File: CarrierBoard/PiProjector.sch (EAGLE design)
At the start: 73 parts, among them P8 PINHEAD2X23, P9 PINHEAD2X23, Q1 BCX70SMD, X1 24MHz, X2 12Mhz

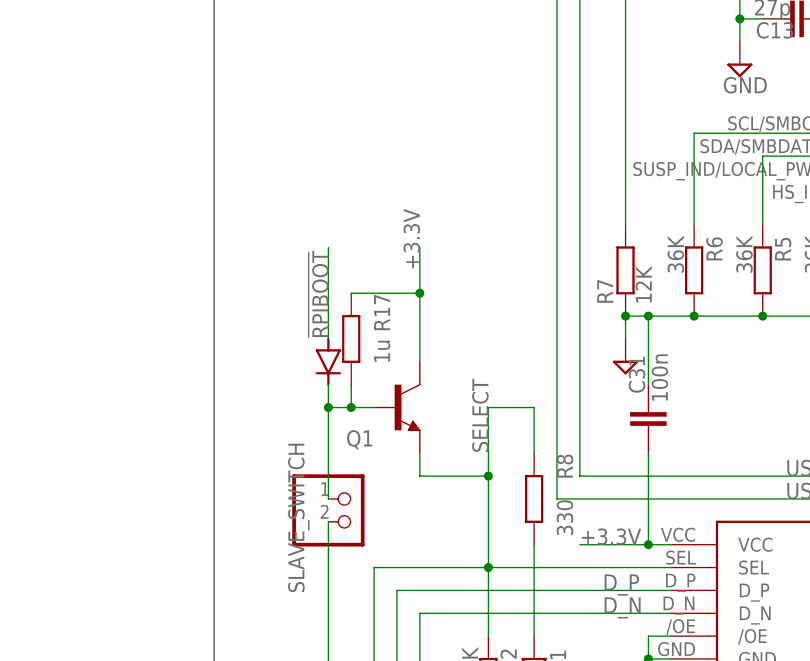
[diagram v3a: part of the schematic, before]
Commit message: Fixed rpiboot
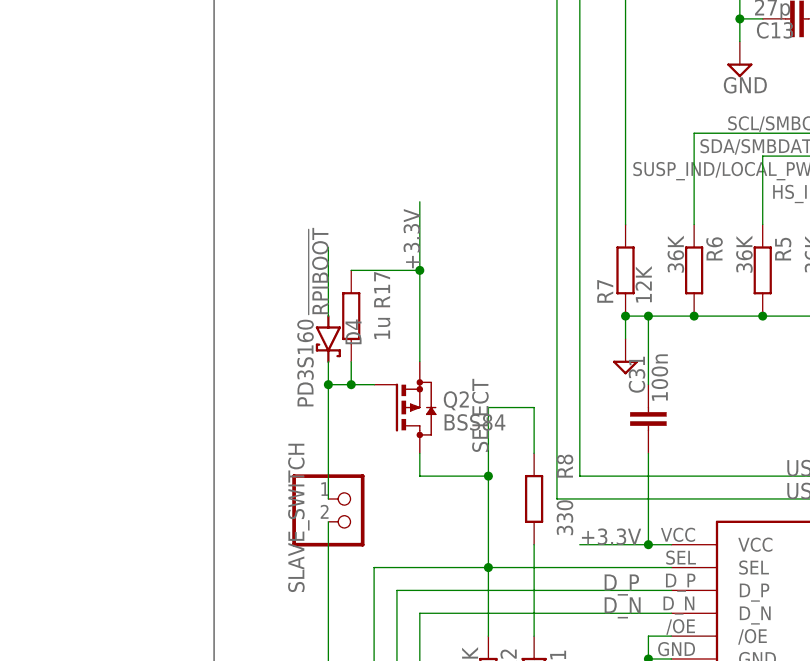
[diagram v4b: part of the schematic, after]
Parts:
- removed Q1: BCX70SMD, transistor-npn:BCX70SMD
- added D4: PD3S160, diode:PD3S160
- added Q2: BSS84, transistor-small-signal:BSS84
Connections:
- net !RPIBOOT: now also D4.A
- net +3.3V: now also Q2.S; no longer Q1.C
- net N$8: now also D4.C, Q2.G; no longer Q1.B
- net SELECT: now also Q2.D; no longer Q1.E
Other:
- moved on the sheet: R17
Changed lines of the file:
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@@
 <part name="SUPPLY29" library="supply2" library_urn="urn:adsk.eagle:library:372" deviceset="GND" device=""/>
 <part name="SUPPLY30" library="supply2" library_urn="urn:adsk.eagle:library:372" deviceset="GND" device=""/>
-<part name="Q1" library="transistor-npn" library_urn="urn:adsk.eagle:library:398" deviceset="BCX70*" device="SMD" package3d_urn="urn:adsk.eagle:package:28738/2"/>
 <part name="R17" library="pm-labs" deviceset="R" device="0603R" value="1u"/>
 <part name="SUPPLY5" library="supply2" library_urn="urn:adsk.eagle:library:372" deviceset="GND" device=""/>
 <part name="SUPPLY22" library="supply2" library_urn="urn:adsk.eagle:library:372" deviceset="GND" device=""/>
-<part name="D3" library="docu-dummy" library_urn="urn:adsk.eagle:library:215" deviceset="DIODE" device=""/>
+<part name="D4" library="diode" library_urn="urn:adsk.eagle:library:210" deviceset="PD3S160" device="" package3d_urn="urn:adsk.eagle:package:43459/1"/>
+<part name="Q2" library="transistor-small-signal" library_urn="urn:adsk.eagle:library:401" deviceset="BSS84" device="" package3d_urn="urn:adsk.eagle:package:28738/2"/>
 </parts>
 <sheets>
@@
 <attribute name="VALUE" x="-45.085" y="210.185" size="1.778" layer="96"/>
 </instance>
-<instance part="Q1" gate="G$1" x="147.32" y="195.58" smashed="yes">
-<attribute name="NAME" x="144.78" y="193.04" size="1.778" layer="95" rot="R180"/>
-</instance>
-<instance part="R17" gate="R" x="142.24" y="203.2" smashed="yes" rot="R270">
-<attribute name="NAME" x="144.78" y="208.28" size="1.778" layer="95" rot="R270"/>
-<attribute name="VALUE" x="144.78" y="203.2" size="1.778" layer="96" rot="R270"/>
+<instance part="R17" gate="R" x="142.24" y="205.74" smashed="yes" rot="R270">
+<attribute name="NAME" x="144.78" y="210.82" size="1.778" layer="95" rot="R270"/>
+<attribute name="VALUE" x="144.78" y="205.74" size="1.778" layer="96" rot="R270"/>
 </instance>
 <instance part="SUPPLY5" gate="GND" x="162.56" y="157.48" smashed="yes">
@@
 <attribute name="VALUE" x="137.795" y="154.305" size="1.778" layer="96"/>
 </instance>
-<instance part="D3" gate="G$1" x="139.7" y="200.66" smashed="yes" rot="R270"/>
+<instance part="D4" gate="G$1" x="139.7" y="203.2" smashed="yes" rot="R270">
+<attribute name="NAME" x="141.605" y="205.486" size="1.778" layer="95" rot="R270"/>
+<attribute name="VALUE" x="136.271" y="205.486" size="1.778" layer="96" rot="R270"/>
+</instance>
+<instance part="Q2" gate="G$1" x="149.86" y="195.58" smashed="yes">
+<attribute name="NAME" x="152.4" y="195.58" size="1.778" layer="95"/>
+<attribute name="VALUE" x="152.4" y="193.04" size="1.778" layer="96"/>
+</instance>
 </instances>
 <busses>
@@
 </segment>
 <segment>
-<pinref part="Q1" gate="G$1" pin="C"/>
-<wire x1="149.86" y1="208.28" x2="149.86" y2="200.66" width="0.1524" layer="91"/>
+<wire x1="149.86" y1="210.82" x2="149.86" y2="200.66" width="0.1524" layer="91"/>
 <pinref part="R17" gate="R" pin="1"/>
-<wire x1="149.86" y1="208.28" x2="142.24" y2="208.28" width="0.1524" layer="91"/>
-<junction x="149.86" y="208.28"/>
-<wire x1="149.86" y1="213.36" x2="149.86" y2="208.28" width="0.1524" layer="91"/>
+<wire x1="149.86" y1="210.82" x2="142.24" y2="210.82" width="0.1524" layer="91"/>
+<junction x="149.86" y="210.82"/>
 <label x="149.86" y="210.82" size="1.778" layer="95" rot="R90"/>
+<pinref part="Q2" gate="G$1" pin="S"/>
+<wire x1="149.86" y1="210.82" x2="149.86" y2="218.44" width="0.1524" layer="91"/>
 </segment>
 </net>
@@
 </segment>
 <segment>
-<wire x1="139.7" y1="203.2" x2="139.7" y2="213.36" width="0.1524" layer="91"/>
-<label x="139.7" y="203.2" size="1.778" layer="95" rot="R90"/>
+<wire x1="139.7" y1="205.74" x2="139.7" y2="213.36" width="0.1524" layer="91"/>
+<label x="139.7" y="205.74" size="1.778" layer="95" rot="R90"/>
+<pinref part="D4" gate="G$1" pin="A"/>
 </segment>
 </net>
@@
 <wire x1="157.48" y1="195.58" x2="157.48" y2="187.96" width="0.1524" layer="91"/>
 <label x="157.48" y="190.5" size="1.778" layer="95" rot="R90"/>
-<pinref part="Q1" gate="G$1" pin="E"/>
 <wire x1="157.48" y1="187.96" x2="157.48" y2="177.8" width="0.1524" layer="91"/>
 <wire x1="149.86" y1="190.5" x2="149.86" y2="187.96" width="0.1524" layer="91"/>
 <wire x1="149.86" y1="187.96" x2="157.48" y2="187.96" width="0.1524" layer="91"/>
 <junction x="157.48" y="187.96"/>
+<pinref part="Q2" gate="G$1" pin="D"/>
 </segment>
 </net>
@@
 <segment>
 <pinref part="R17" gate="R" pin="2"/>
-<wire x1="142.24" y1="198.12" x2="142.24" y2="195.58" width="0.1524" layer="91"/>
-<pinref part="Q1" gate="G$1" pin="B"/>
-<wire x1="142.24" y1="195.58" x2="144.78" y2="195.58" width="0.1524" layer="91"/>
-<wire x1="142.24" y1="195.58" x2="139.7" y2="195.58" width="0.1524" layer="91"/>
-<wire x1="139.7" y1="195.58" x2="139.7" y2="185.42" width="0.1524" layer="91"/>
-<junction x="142.24" y="195.58"/>
+<wire x1="142.24" y1="200.66" x2="142.24" y2="198.12" width="0.1524" layer="91"/>
+<wire x1="142.24" y1="198.12" x2="144.78" y2="198.12" width="0.1524" layer="91"/>
+<wire x1="142.24" y1="198.12" x2="139.7" y2="198.12" width="0.1524" layer="91"/>
+<wire x1="139.7" y1="198.12" x2="139.7" y2="185.42" width="0.1524" layer="91"/>
+<junction x="142.24" y="198.12"/>
 <pinref part="SLAVE_SWITCH" gate="G$1" pin="1"/>
-<wire x1="139.7" y1="195.58" x2="139.7" y2="198.12" width="0.1524" layer="91"/>
-<junction x="139.7" y="195.58"/>
-</segment>
-</net>
+<wire x1="139.7" y1="198.12" x2="139.7" y2="200.66" width="0.1524" layer="91"/>
+<junction x="139.7" y="198.12"/>
+<pinref part="D4" gate="G$1" pin="C"/>
+<pinref part="Q2" gate="G$1" pin="G"/>
+</segment>
+</net>

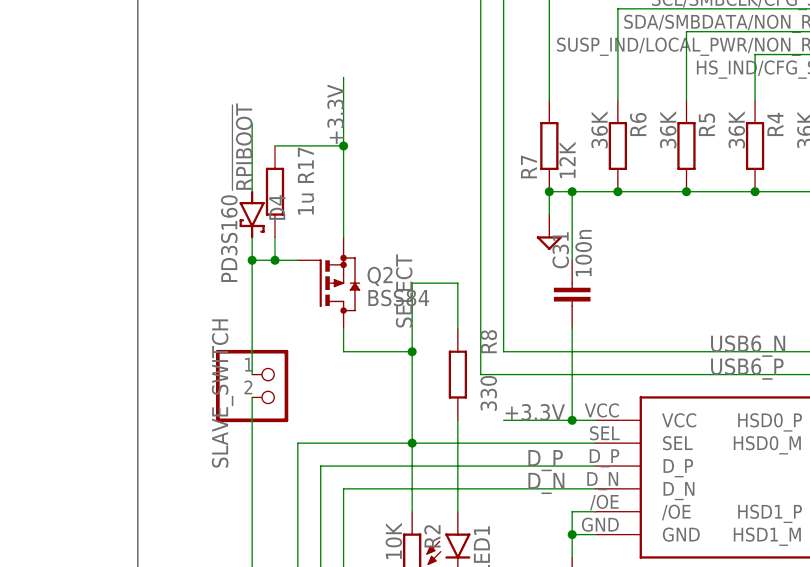
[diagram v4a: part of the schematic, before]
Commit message: Fixed RPI and USB switch Pulldown
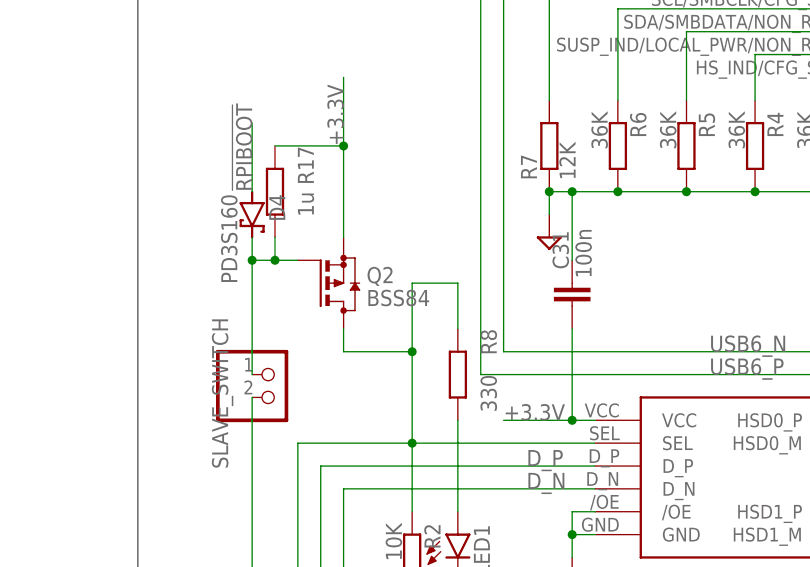
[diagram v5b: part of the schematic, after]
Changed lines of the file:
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@@
 <wire x1="157.48" y1="195.58" x2="162.56" y2="195.58" width="0.1524" layer="91"/>
 <wire x1="157.48" y1="195.58" x2="157.48" y2="187.96" width="0.1524" layer="91"/>
-<label x="157.48" y="190.5" size="1.778" layer="95" rot="R90"/>
 <wire x1="157.48" y1="187.96" x2="157.48" y2="177.8" width="0.1524" layer="91"/>
 <wire x1="149.86" y1="190.5" x2="149.86" y2="187.96" width="0.1524" layer="91"/>

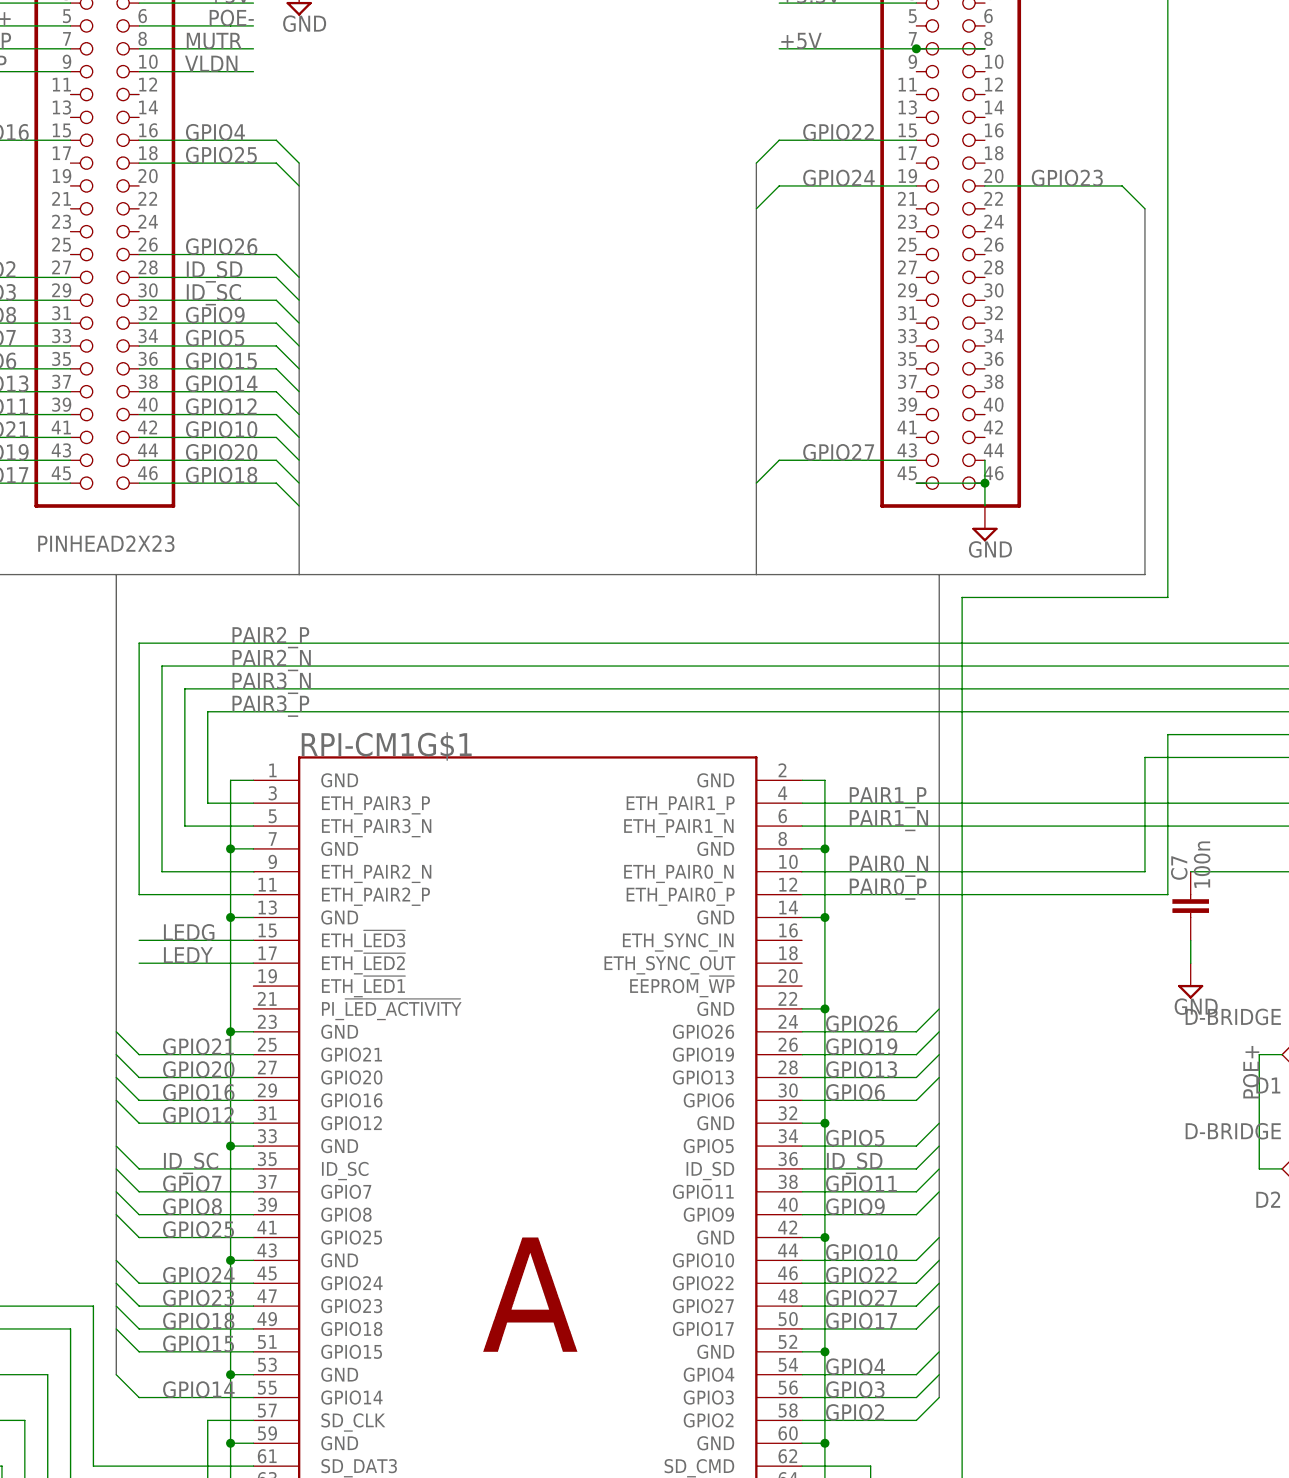
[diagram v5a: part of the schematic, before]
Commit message: Added an I2C expander
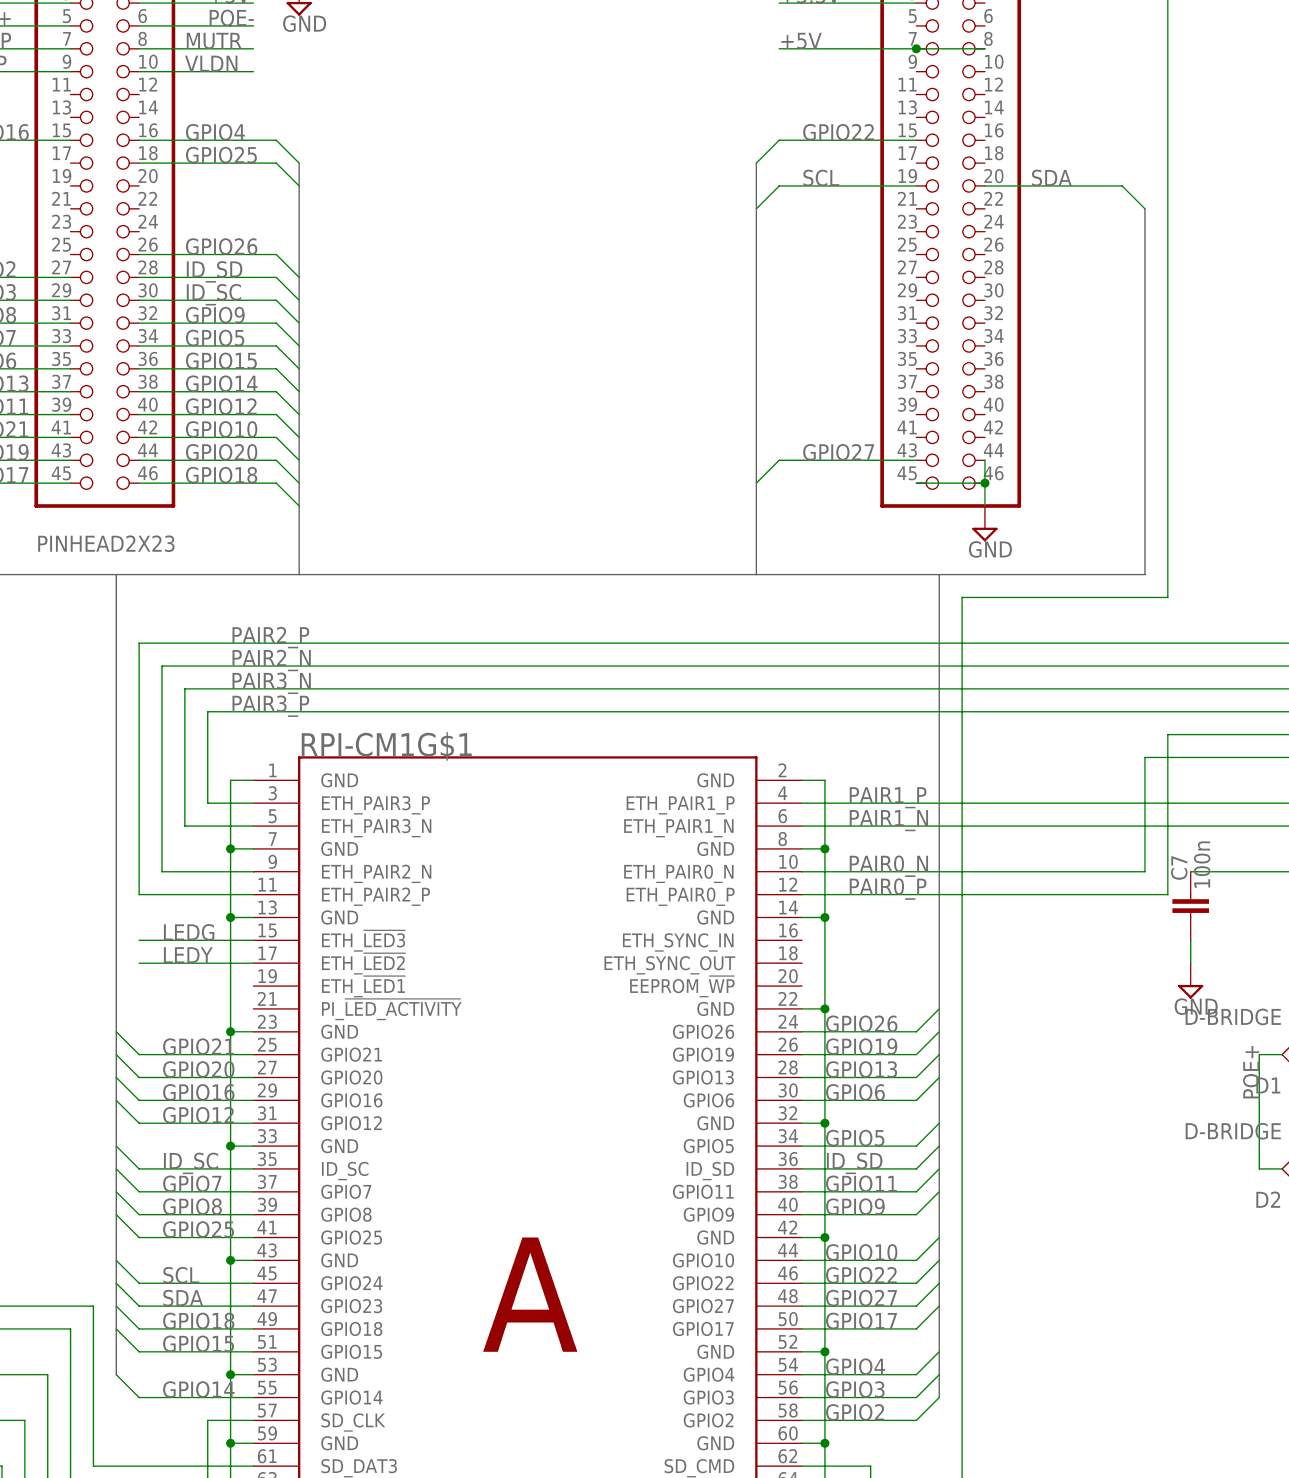
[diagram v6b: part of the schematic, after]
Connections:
- net GPIO23 renamed SDA
- net GPIO24 renamed SCL
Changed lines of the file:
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@@
 </segment>
 </net>
-<net name="GPIO23" class="0">
+<net name="SDA" class="0">
 <segment>
 <pinref part="P9" gate="G$1" pin="20"/>
@@
 </segment>
 </net>
-<net name="GPIO24" class="0">
+<net name="SCL" class="0">
 <segment>
 <pinref part="P9" gate="G$1" pin="19"/>
